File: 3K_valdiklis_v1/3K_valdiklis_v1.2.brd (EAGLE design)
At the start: 120 x 90 mm, 66 parts, among them IC2 L293D, IC4 ATMEGA1284, IC5 DS1307, J4 HEAD3X2, K1 S202T02, K2 S202T02, K3 S202T02, K4 S202T02, K5 S202T02, K6 S202T02, Q4 32.768, T2 TIP120V, X1 Boiler pump, X10 22-23-2031, X11 +12V, X2 Storage tank pump, X3 Radiator pump, X4 4 way valve 1, X5 4 way valve 2, X6 Floor heating, X7 motorized valve 1, X77 PUMP1, X8 motorized valve 2, X9 16MHz, Y1 12mhz

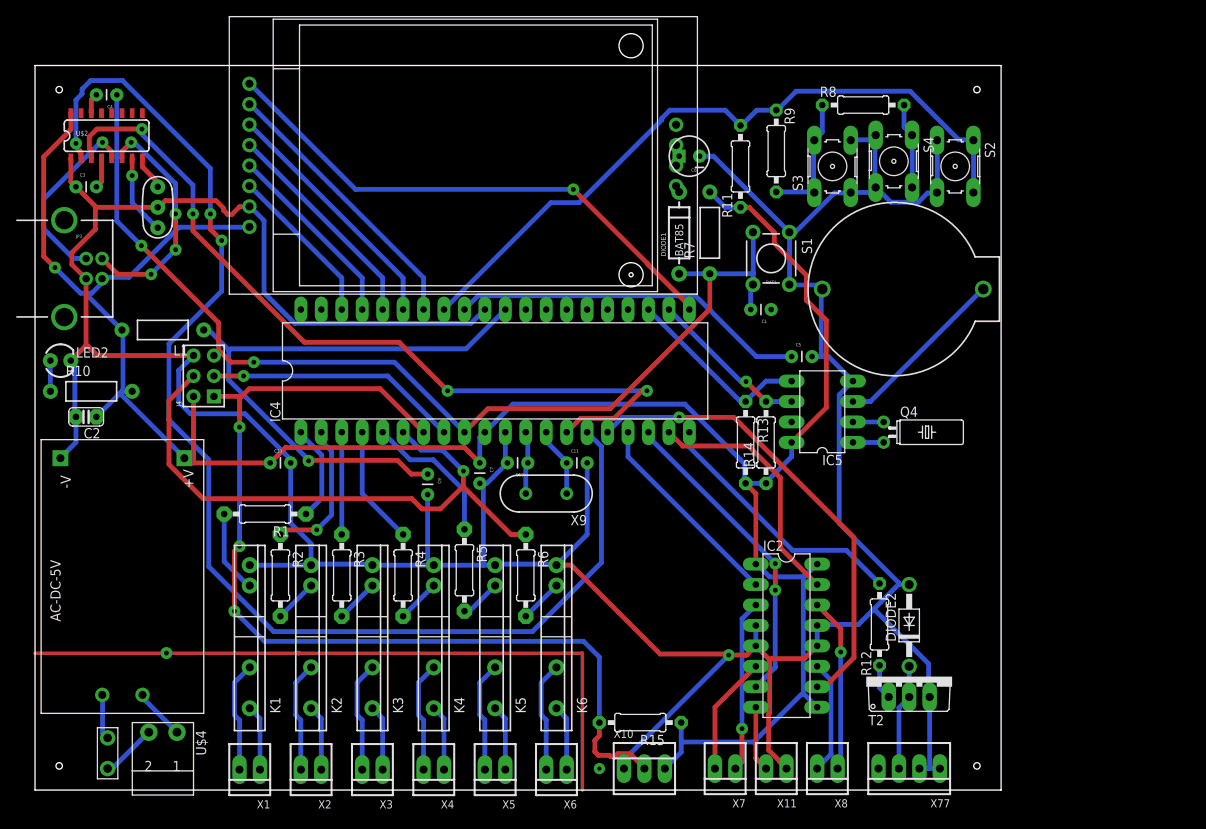
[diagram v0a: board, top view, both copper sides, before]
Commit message: TRASAvimas
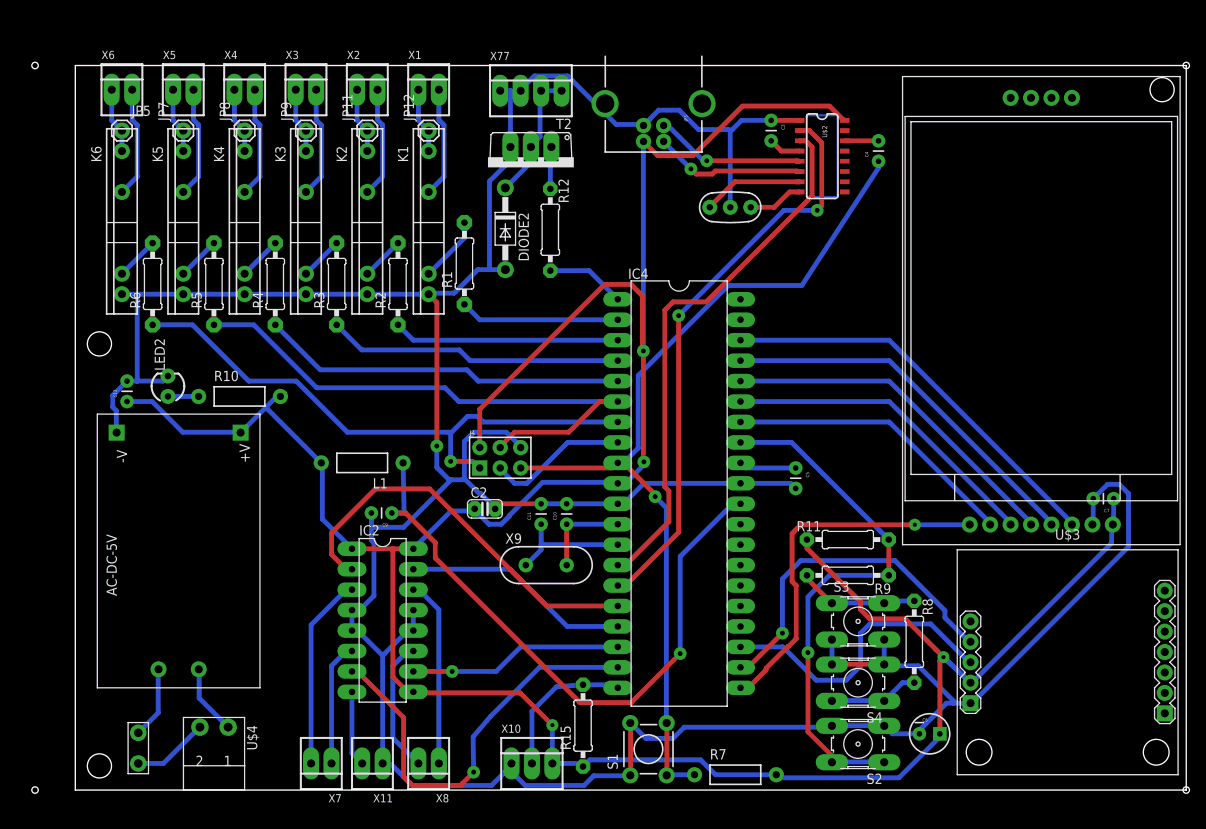
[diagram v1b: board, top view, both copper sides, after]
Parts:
- removed BAT1: (no value), SparkFun-Electromechanical:BATTCOM_20MM_PTH
- removed C1: 22p, SparkFun:CAP-PTH-SMALL
- removed DIODE1: BAT85, SteveMarple:DIODE-TH-0.4
- removed IC5: DS1307, adafruit:DIL08
- removed Q4: 32.768, crystal:TC38H
- removed R13: 2.2k, adafruit:0207/10
- removed R14: 2.2K, adafruit:0207/10
- added JP11, JP12, JP5, JP7, JP8, JP9: M01PTH, SparkFun-Connectors-1:1X01
- added U$3: RTC-EEPROM-BATTERY, diy-modules-1:RTC_EEPROM_BATTERY
- moved U$1 122.1 mm to (142.2, 30.5), turned to 90 degrees
- moved X6 100.2 mm to (10.8, 87.0), turned to 0 degrees
- moved X77 96.4 mm to (61.6, 86.9), turned to 0 degrees
- moved C4 95.0 mm to (104.8, 78.1), turned to 90 degrees
- moved X5 92.9 mm to (18.4, 87.0), turned to 0 degrees
- moved U$2 88.9 mm to (97.8, 78.7), turned to 270 degrees
- moved X4 87.7 mm to (26.0, 87.0), turned to 0 degrees
- moved X1 87.3 mm to (48.9, 87.0), turned to 0 degrees
- moved C3 86.8 mm to (91.4, 83.2), turned to 270 degrees
- moved X3 84.9 mm to (33.7, 87.0), turned to 0 degrees
- moved X2 84.7 mm to (41.3, 87.0), turned to 0 degrees
- moved K6 80.0 mm to (10.8, 74.3), turned to 270 degrees
- moved C7 78.9 mm to (134.0, 36.2), turned to 180 degrees
- moved T2 78.8 mm to (61.6, 77.3), turned to 180 degrees
- moved C6 77.7 mm to (111.1, 6.99), turned to 0 degrees
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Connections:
- removed net DTR: C1.1
- removed net N$15: DIODE2.C, T2.C, X77.3
- removed net N$20: IC5.1, Q4.2
- removed net N$21: IC5.2, Q4.1
- removed net N$27: BAT1.1, IC5.3
- removed net SQW: IC5.7
- new net GND.2: U$3.J2.2
- new net N$40: U$3.J1.5
- new net VCC.2: U$3.J2.3
- net !RESET: no longer C1.2, DIODE1.A
- net +12V: now also DIODE2.C, T2.C, X77.3
- net D0: now also R12.1; no longer R1.1
- net D1: now also R1.1; no longer R2.1
- net D10(RX1): now also IC2.2; no longer IC2.10
- net D11(TX1): now also IC2.15; no longer IC2.2
- net D12: now also IC2.10; no longer IC2.7
- net D13: now also IC2.7; no longer IC2.15
- net D14: now also R15.2, X10.2; no longer R12.1
- net D16(SCL): now also U$3.J1.4; no longer IC5.6, R14.2
- net D17(SDA): now also U$3.J1.3; no longer IC5.5, R13.1
- net D2: now also R2.1; no longer R3.1
- net D3: now also R3.1; no longer R4.1
- net D4: now also R4.1; no longer R5.1
- net D5(MOSI): now also R5.1; no longer R6.1
- net D6(MISO): now also R6.1; no longer R15.2, X10.2
- net GND: now also U$3.J1.1; no longer BAT1.2, IC5.4
- net MV1.1: now also X7.2; no longer X7.1
- net MV1.2: now also X7.1; no longer X7.2
- net N$18: now also JP9.1
- net N$25: now also JP11.1
- net N$29: now also JP8.1
- net N$32: now also JP12.1
- net N$35: now also JP5.1
- net N$38: now also JP7.1
- net VCC: now also U$3.J1.2; no longer DIODE1.C, IC5.8, R13.2, R14.1
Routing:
- net N$17: track 170.1 -> 0.00 mm, vias 1 -> 0
- net D9(TX0): track 157.5 -> 71.8 mm, vias 3 -> 2
- net VCC: track 281.7 -> 363.7 mm, vias 1 -> 4
- net D6(MISO): track 122.6 -> 71.9 mm, vias 3 -> 1
- net AREF: track 44.5 -> 7.12 mm
- net D8(RX0): track 101.7 -> 67.2 mm, vias 4 -> 0
- net A2: track 20.1 -> 50.8 mm
- net D4: track 17.9 -> 45.4 mm
- net N$20: track 3.81 -> 27.9 mm
- net A3: track 23.7 -> 47.2 mm
- net D16(SCL): track 20.0 -> 42.7 mm
- net N$27: track 22.0 -> 0.00 mm
- net D3: track 14.8 -> 36.8 mm
- net D15: track 66.6 -> 45.4 mm
- net D13: track 31.3 -> 52.1 mm, vias 0 -> 1
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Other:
- board size 120 x 90 mm -> 138 x 90 mm
